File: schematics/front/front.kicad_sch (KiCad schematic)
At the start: 27 parts, among them J1 USB_B_Micro, J2 MOTOR, J3 DEBUG_UART, J4 RGB, J5 THERMO, SW1 RESET, SW2 BOOT, SW3 MODE, U1 ME6211C33M5, U2 ESP32-S2-MINI-2-N4, U3 DRV8836

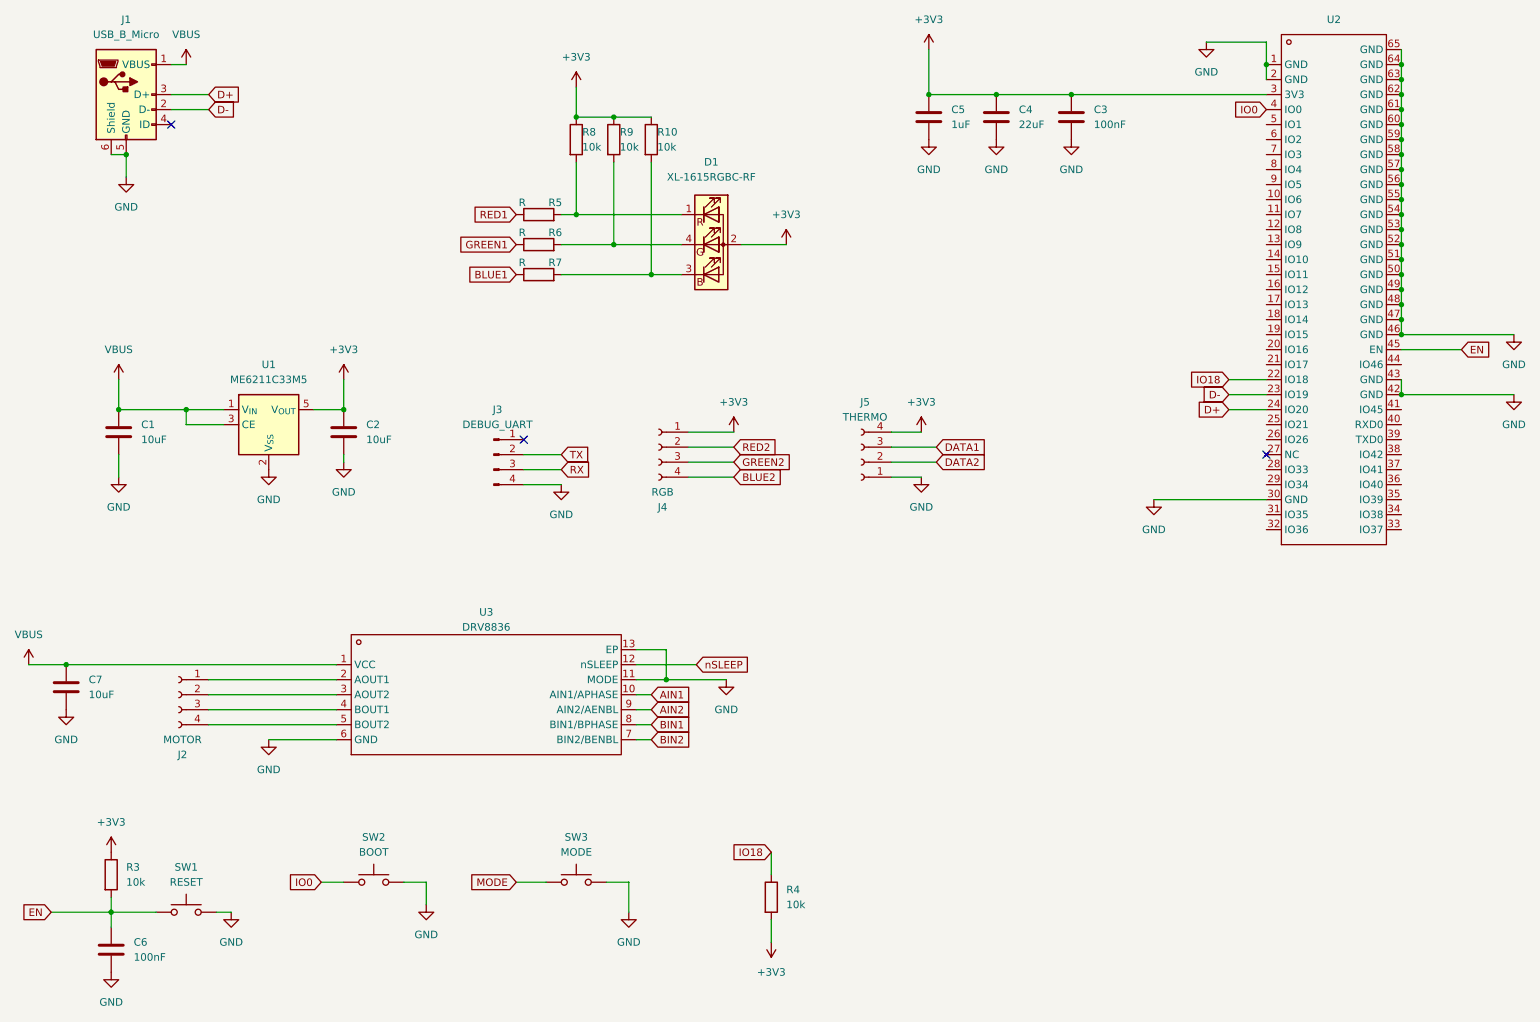
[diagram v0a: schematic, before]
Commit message: Signed-off-by: Ray33ee <30669752+ray33ee@users.noreply.github.com>
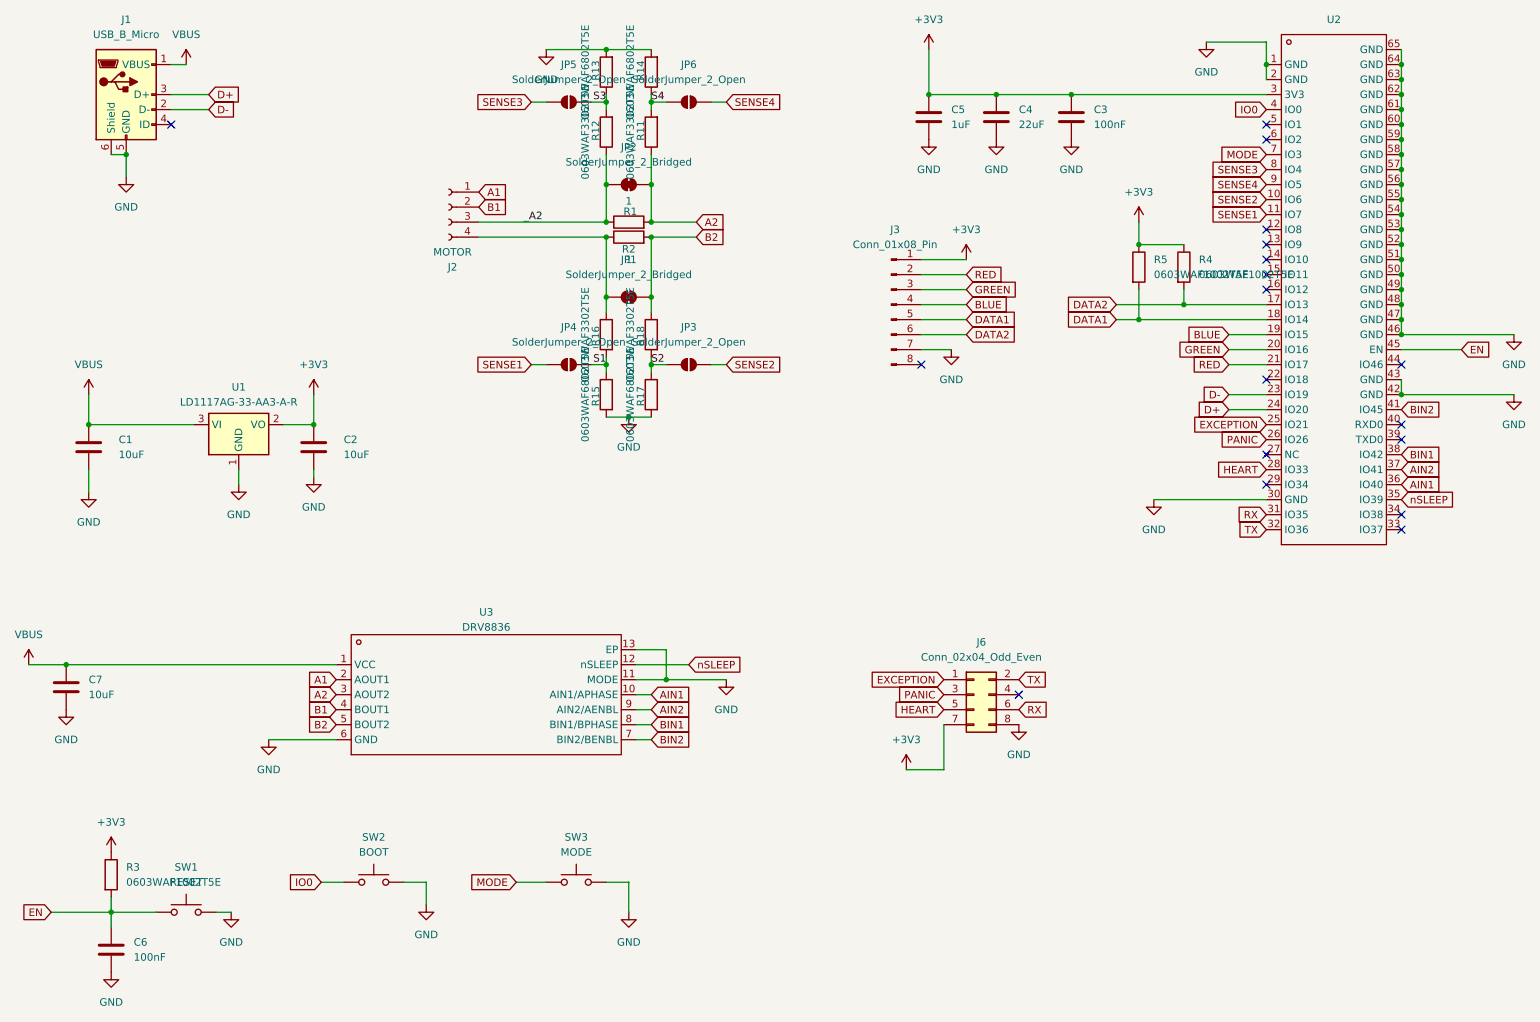
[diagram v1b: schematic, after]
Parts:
- removed D1: XL-1615RGBC-RF, Resistor_SMD:R_Array_Convex_2x0606, symbol Device:LED_RABG
- removed J3: DEBUG_UART, Connector_PinHeader_2.54mm:PinHeader_1x04_P2.54mm_Vertical, symbol Connector:Conn_01x04_Pin
- removed J4: RGB, Connector_JST:JST_SH_SM04B-SRSS-TB_1x04-1MP_P1.00mm_Horizontal, symbol Connector:Conn_01x04_Socket
- removed J5: THERMO, Connector_JST:JST_SH_SM04B-SRSS-TB_1x04-1MP_P1.00mm_Horizontal, symbol Connector:Conn_01x04_Socket
- removed R10, R8, R9: 10k, Resistor_SMD:R_0603_1608Metric, symbol Device:R
- removed R6, R7: R, Resistor_SMD:R_1206_3216Metric, symbol Device:R
- removed U1: ME6211C33M5, Package_TO_SOT_SMD:SOT-23-5, symbol Regulator_Linear:ME6211C33M5
- added J3: Conn_01x08_Pin, connector:SAMTEC-MMT-108-02-X-SH, symbol Connector:Conn_01x08_Pin
- added J6: Conn_02x04_Odd_Even, connector:SAMTEC_CLT-104-02-F-D-BE-K-TR, symbol Connector_Generic:Conn_02x04_Odd_Even
- added JP1, JP2: SolderJumper_2_Bridged, Jumper:SolderJumper-2_P1.3mm_Bridged_RoundedPad1.0x1.5mm, symbol Jumper:SolderJumper_2_Bridged
- added JP3, JP4, JP5, JP6: SolderJumper_2_Open, Jumper:SolderJumper-2_P1.3mm_Open_RoundedPad1.0x1.5mm, symbol Jumper:SolderJumper_2_Open
- added R1, R2: 1, Resistor_SMD:R_1206_3216Metric_Pad1.30x1.75mm_HandSolder, symbol Device:R
- added R11, R12, R16, R18: 0603WAF3302T5E, Resistor_SMD:R_0603_1608Metric, symbol Device:R
- added R13, R14, R15, R17: 0603WAF6802T5E, Resistor_SMD:R_0603_1608Metric, symbol Device:R
- added U1: LD1117AG-33-AA3-A-R, Package_TO_SOT_SMD:SOT-223-3_TabPin2, symbol Regulator_Linear:LD1117S33TR_SOT223
- R3: value 10k -> 0603WAF1002T5E
- R4: value 10k -> 0603WAF1002T5E; footprint Resistor_SMD:R_1206_3216Metric -> Resistor_SMD:R_0603_1608Metric
- R5: value R -> 0603WAF1002T5E; footprint Resistor_SMD:R_1206_3216Metric -> Resistor_SMD:R_0603_1608Metric
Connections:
- net RED1 is gone; now on net +3V3: R5.1
- net +3V3: now also R4.1, J3.1 (Pin_1), J6.7 (Pin_7), U1.2 (VO); no longer R4.2
- net AIN1: now also U2.36 (IO40)
- net AIN2: now also U2.37 (IO41)
- net BIN1: now also U2.38 (IO42)
- net BIN2: now also U2.41 (IO45)
- net DATA1: now also R5.2, U2.18 (IO14), J3.5 (Pin_5)
- net DATA2: now also R4.2, U2.17 (IO13), J3.6 (Pin_6)
- net GND: now also J3.7 (Pin_7), J6.8 (Pin_8), R13.2, R14.2, R15.2, R17.2, U1.1 (GND)
- net MODE: now also U2.7 (IO3)
- net RX: now also U2.31 (IO35), J6.6 (Pin_6)
- net TX: now also U2.32 (IO36), J6.2 (Pin_2)
- net VBUS: now also U1.3 (VI)
- net nSLEEP: now also U2.35 (IO39)
- net A1: now reaches J2.1 (Pin_1), U3.2 (AOUT1)
- net A2: now reaches U3.3 (AOUT2)
- net A2: now also JP2.2 (B), R1.2, R11.1; no longer J2.2 (Pin_2)
- net B1: now reaches U3.4 (BOUT1)
- net B1: now also J2.2 (Pin_2); no longer J2.3 (Pin_3)
- net at J2.4 (Pin_4): now also JP1.1 (A), R16.1, R2.1; no longer U3.5 (BOUT2)
- net SENSE2: now reaches U2.10 (IO6)
- net SENSE2: now also JP3.2 (B)
- net SENSE1: now reaches U2.11 (IO7)
- net SENSE1: now also JP4.1 (A)
- net BLUE: now reaches U2.19 (IO15)
- net BLUE: now also J3.4 (Pin_4)
- net GREEN: now reaches U2.20 (IO16)
- net GREEN: now also J3.3 (Pin_3)
- net RED: now reaches U2.21 (IO17)
- net RED: now also J3.2 (Pin_2)
- net EXCEPTION: now reaches U2.25 (IO21)
- net EXCEPTION: now also J6.1 (Pin_1)
- net PANIC: now reaches U2.26 (IO26)
- net PANIC: now also J6.3 (Pin_3)
- net HEART: now reaches U2.28 (IO33)
- net HEART: now also J6.5 (Pin_5)
- net SENSE3: now reaches U2.8 (IO4)
- net SENSE3: now also JP5.1 (A)
- net SENSE4: now reaches U2.9 (IO5)
- net SENSE4: now also JP6.2 (B)
- net IO18: no longer names the net of U2.22 (IO18)
- net IO18: no longer R4.1
- new net B2: JP1.2 (B), R18.1, R2.2, U3.5 (BOUT2)
- new net S1: JP4.2 (B), R15.1, R16.2
- new net S2: JP3.1 (A), R17.1, R18.2
- new net S3: JP5.2 (B), R12.2, R13.1
- new net S4: JP6.1 (A), R11.2, R14.1
- new net _A2: J2.3 (Pin_3), JP2.1 (A), R1.1, R12.1
- no-connect marks 3 -> 18
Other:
- moved on the sheet: J2
